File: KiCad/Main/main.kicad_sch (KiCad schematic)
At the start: 15 parts, among them J3 Vers Display, J8 RJ45, SW2 SW_DPST_x2, SW3 SW_DPST, SW4 SW_DPST_x2, U5 ESP32-S3-DevKitC

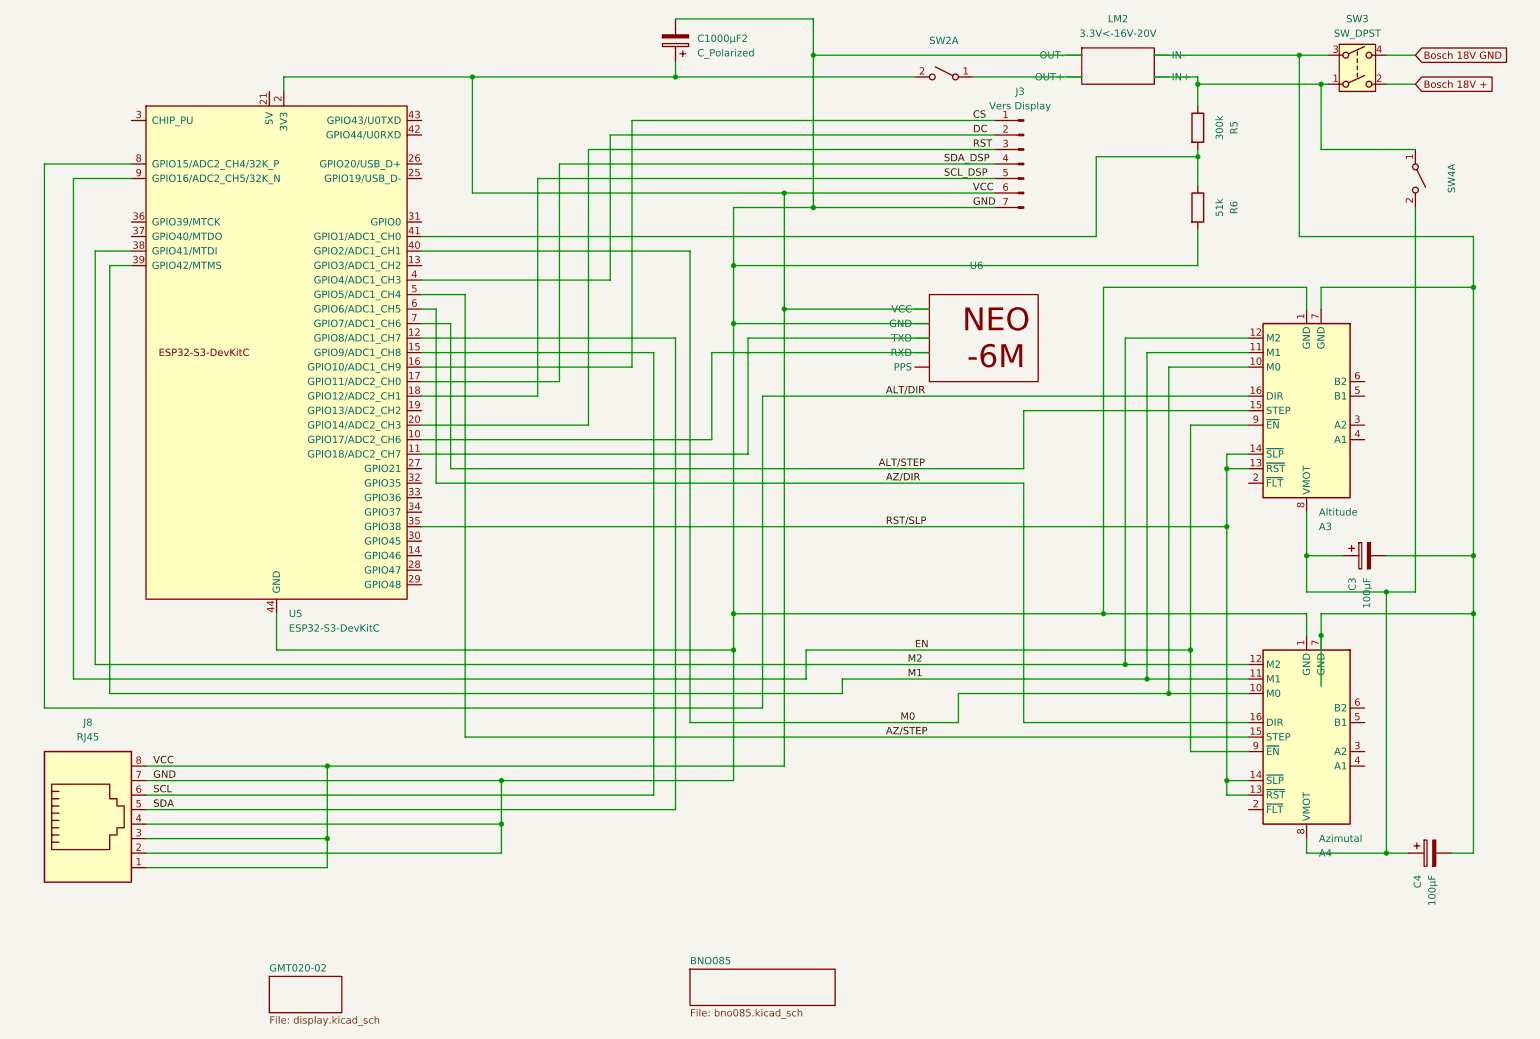
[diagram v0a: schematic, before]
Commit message: bno085 et moteurs OK
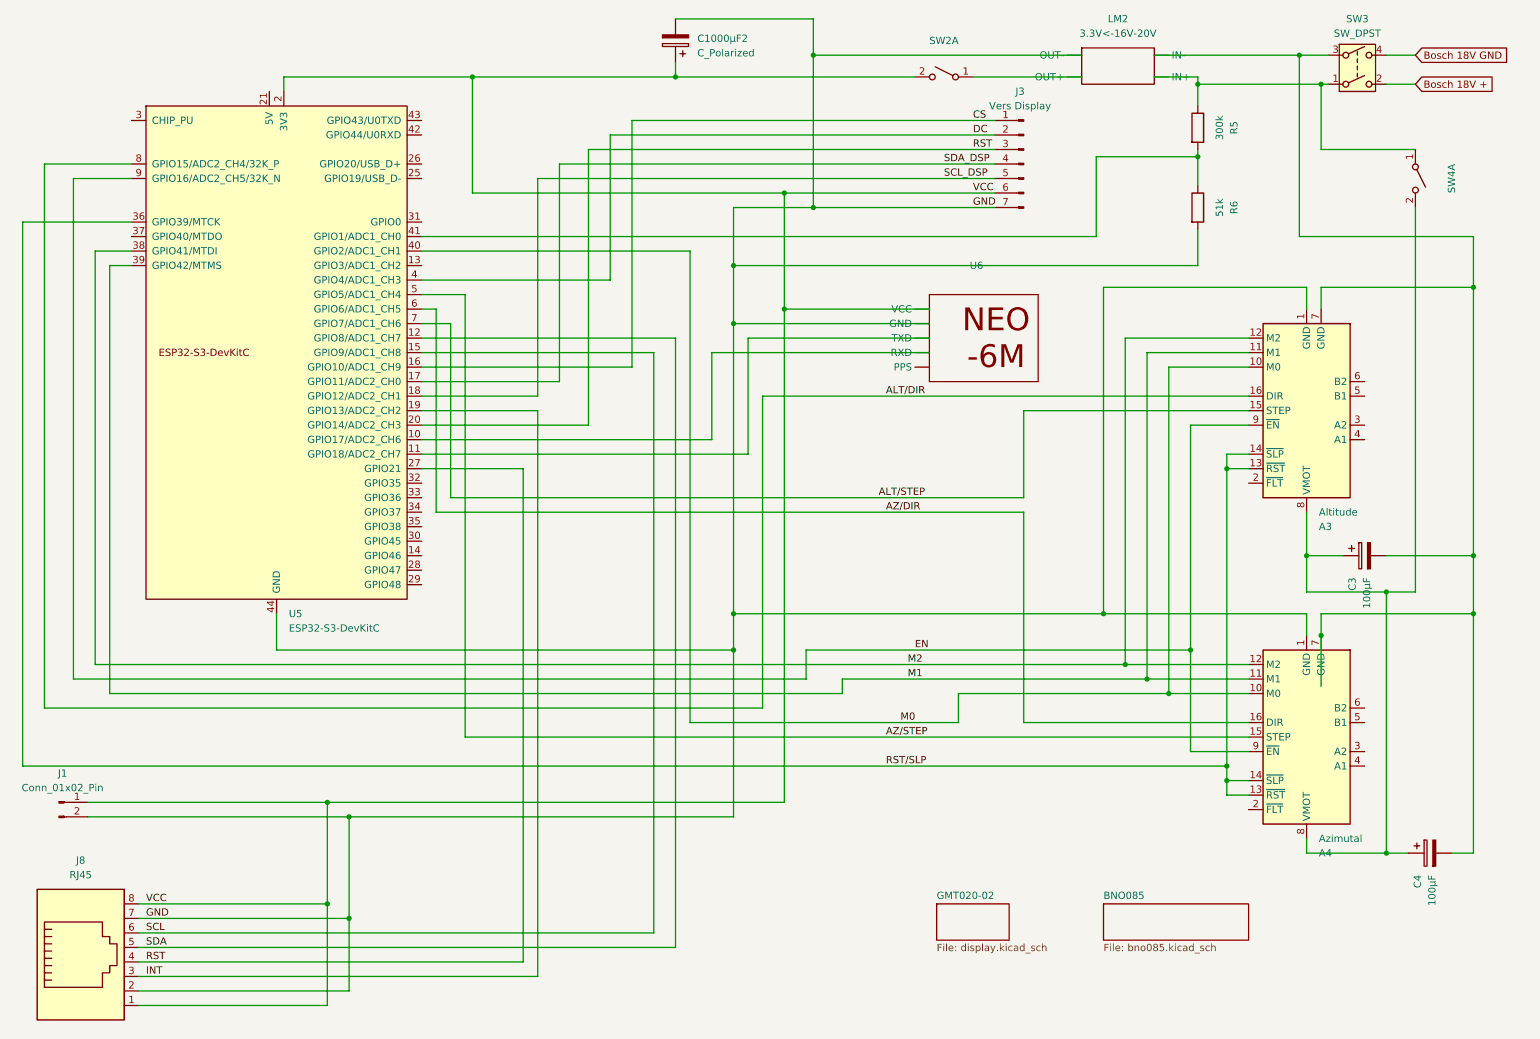
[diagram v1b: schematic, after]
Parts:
- added J1: Conn_01x02_Pin, symbol Connector:Conn_01x02_Pin
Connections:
- net GND: now also J1.2 (Pin_2); no longer J8.4
- net RST: now also J8.4, U5.27 (GPIO21)
- net RST/SLP: now also U5.36 (GPIO39/MTCK); no longer U5.35 (GPIO38)
- net VCC: now also J1.1 (Pin_1); no longer J8.3
- net INT: now reaches U5.19 (GPIO13/ADC2_CH2)
- net INT: now also J8.3
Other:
- moved on the sheet: J8
